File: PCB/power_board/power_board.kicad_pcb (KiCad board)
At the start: 4 copper layers, 73 x 73 mm, 74 parts, among them IC1 TPS61131PW, IC11 TPS61032PWP, IC7 BQ51013BRHLR, IC9 MAX17048G+T10, J1 Speaker_con, J2 DS1013-40SSIB1-B-0, J3 USB4110GFA, J4 IMU_connector, J6 ACCEL_connector, Q2 Si2323DDS-T1-GE3, Q3 BSS138, U2 MCP73871-2CA

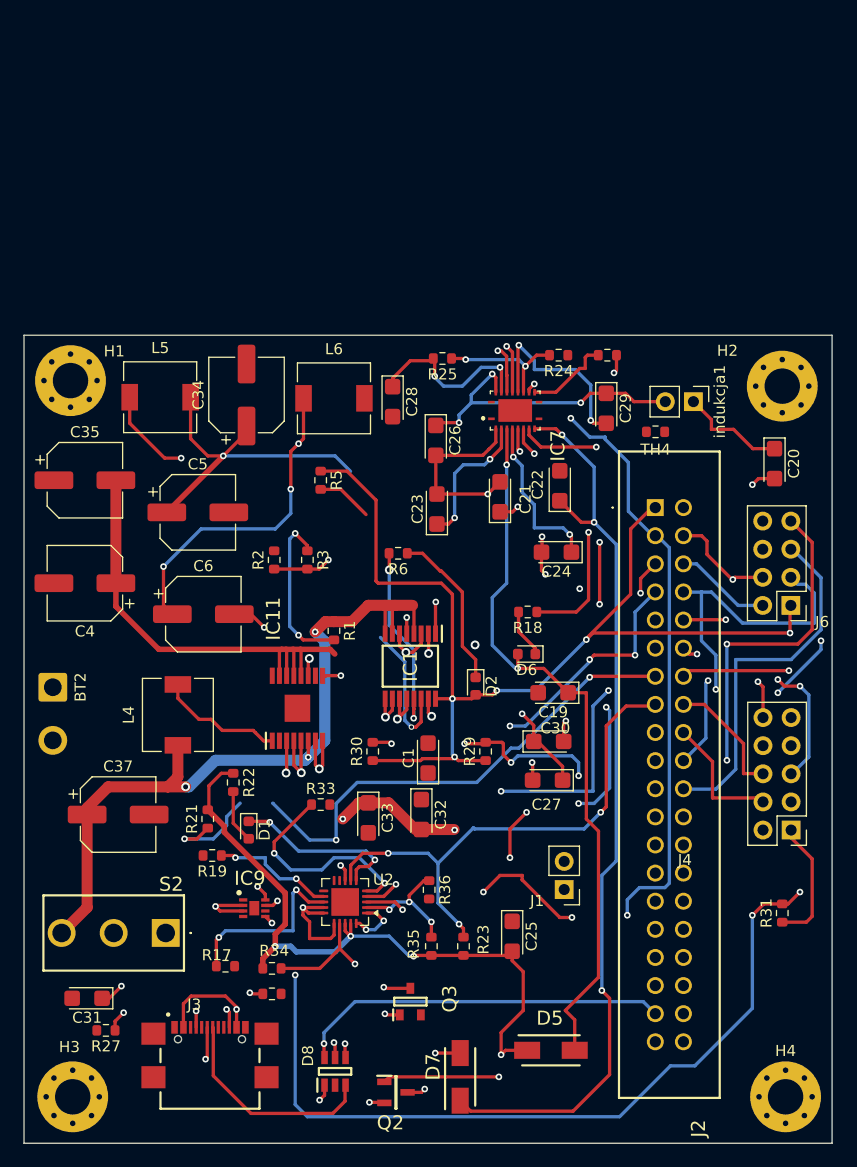
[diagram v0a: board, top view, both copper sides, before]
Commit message: modified gnd
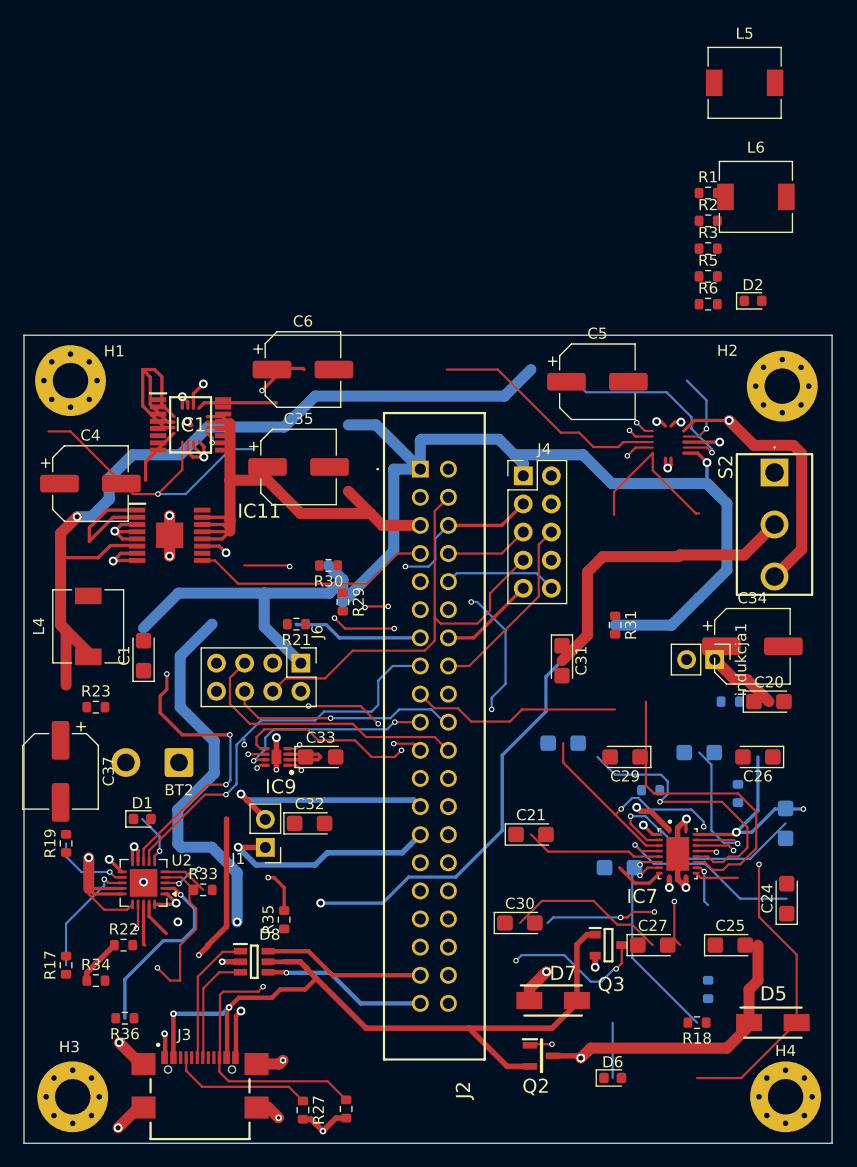
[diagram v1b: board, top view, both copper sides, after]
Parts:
- C19, C22, C23, C28, R20, R24, R25, TH4: moved to B.Cu
- moved S2 69.0 mm to (96.0, 111.3), turned to -90 degrees
- moved L5 60.0 mm to (93.3, 76.1)
- moved C31 52.6 mm to (76.8, 128.3), turned to -90 degrees
- moved R1 52.0 mm to (90.0, 86.1), turned to 0 degrees
- moved C34 51.0 mm to (94.0, 127.0), turned to 0 degrees
- moved TH4 50.6 mm to (90.0, 158.0), turned to 90 degrees
- moved R2 49.8 mm to (90.0, 88.6), turned to 0 degrees
- moved R3 45.8 mm to (90.0, 91.1), turned to 0 degrees
- moved J6 44.6 mm to (53.2, 128.5), turned to -90 degrees
- moved R25 43.3 mm to (84.8, 140.0)
- moved D2 42.9 mm to (94.1, 95.8), turned to 0 degrees
- moved IC7 42.4 mm to (87.2, 145.4), turned to 0 degrees
- moved C23 42.4 mm to (97.0, 143.0)
- moved L6 42.2 mm to (94.3, 86.4)
- moved C28 42.1 mm to (89.2, 136.6), turned to 180 degrees
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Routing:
- net GND: track 29.9 -> 130.2 mm, vias 8 -> 37
- net (no net): track 0.00 -> 92.1 mm, vias 0 -> 3
- net Net-(IC7-~{AD-EN}): track 90.3 -> 23.3 mm, vias 6 -> 2
- net /FG_ALRT: track 104.3 -> 41.2 mm, vias 4 -> 1
- net /USB_SRC: track 82.5 -> 19.9 mm, vias 3 -> 1
- net Net-(IC1-SWN): track 52.0 -> 0.00 mm, vias 3 -> 0
- net unconnected-(J2-Pad2): track 0.00 -> 51.2 mm, vias 0 -> 1
- net /CHARGER_SRC: track 71.6 -> 119.9 mm, vias 5 -> 3
- net Net-(IC1-SWP): track 56.3 -> 12.8 mm, vias 4 -> 2
- net Net-(S2-COM): track 38.1 -> 80.7 mm, vias 3 -> 2
- net /I2C_SDA: track 64.8 -> 22.2 mm, vias 6 -> 2
- net /V_SYS: track 99.9 -> 141.4 mm, vias 4 -> 2
- net Net-(IC7-CLAMP2): track 48.7 -> 12.7 mm
- net Net-(Q3-D): track 13.9 -> 48.8 mm, vias 2 -> 4
- net /BAT+: track 95.6 -> 65.1 mm, vias 4 -> 1
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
